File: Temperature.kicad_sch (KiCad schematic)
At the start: 14 parts, among them U4 LMV324

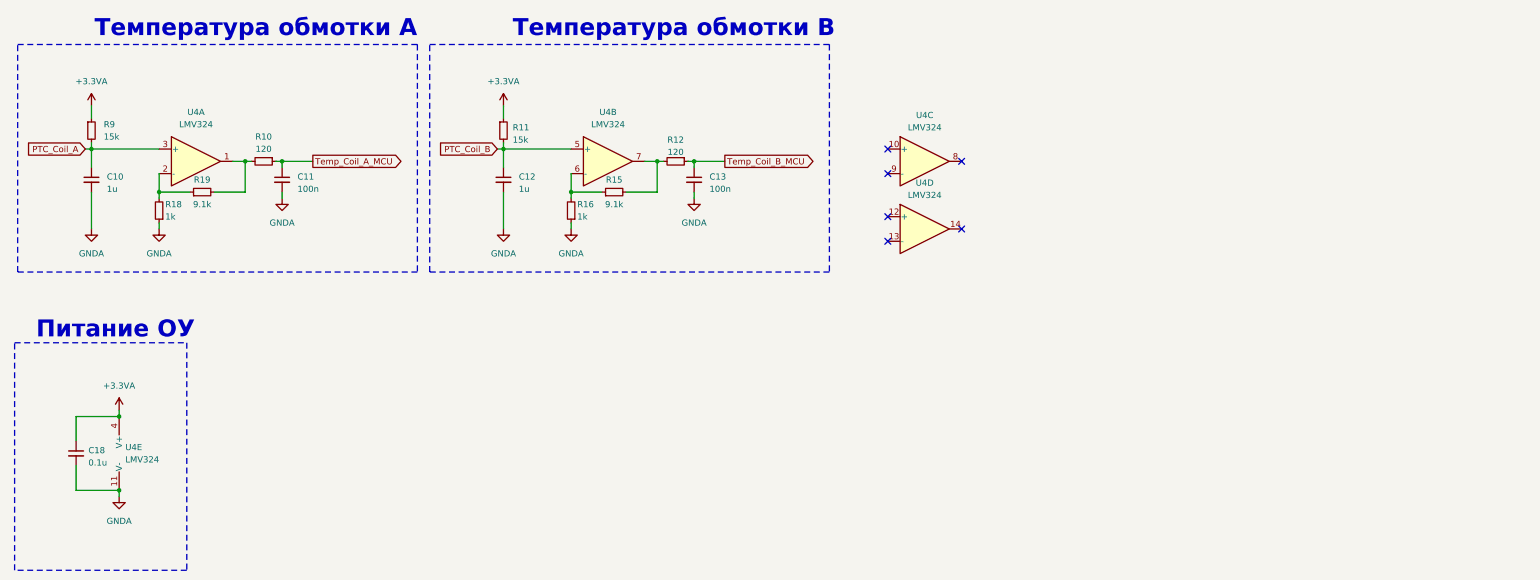
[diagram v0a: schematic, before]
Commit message: Изменения: добавил папку с отчетностью
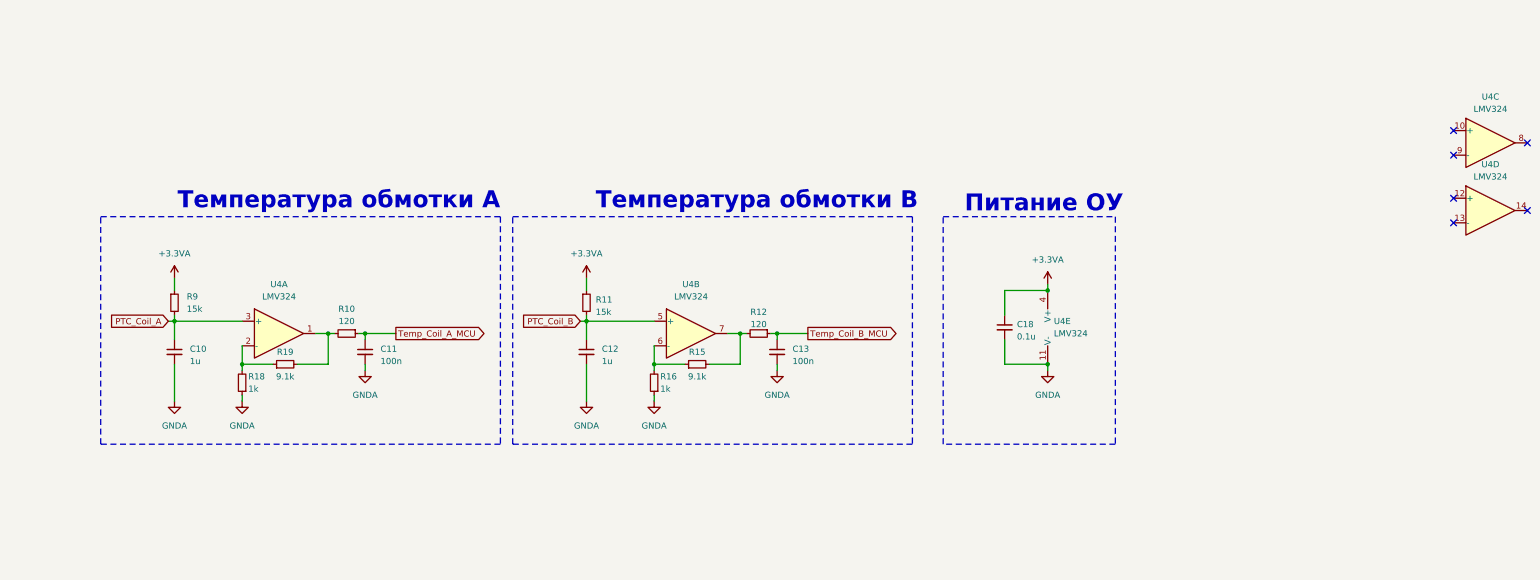
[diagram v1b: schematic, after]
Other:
- moved on the sheet: C10, C11, C12, C13, C18, R10, R11, R12, R15, R16, R18, R19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
